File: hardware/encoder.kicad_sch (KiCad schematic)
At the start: 9 parts, among them SW2 PEC12R Encoder

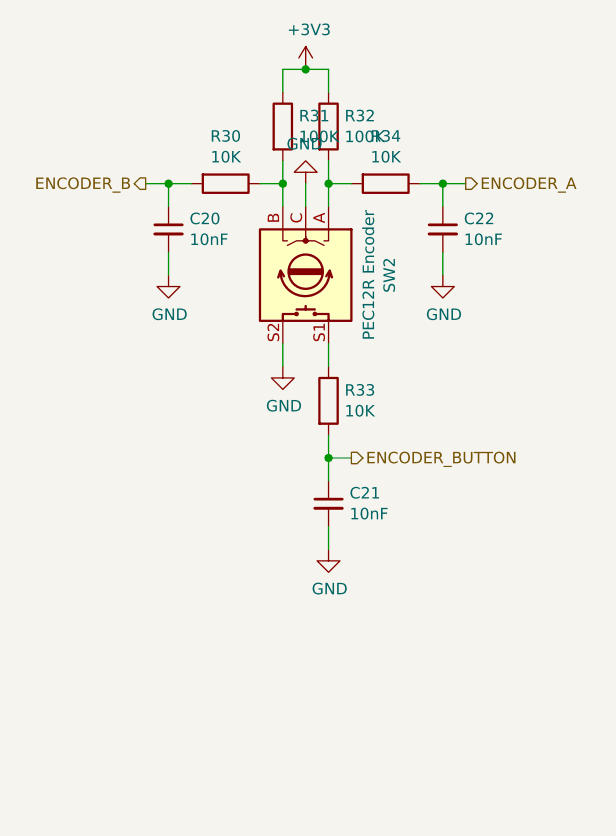
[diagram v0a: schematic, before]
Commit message: Major changes to schematic
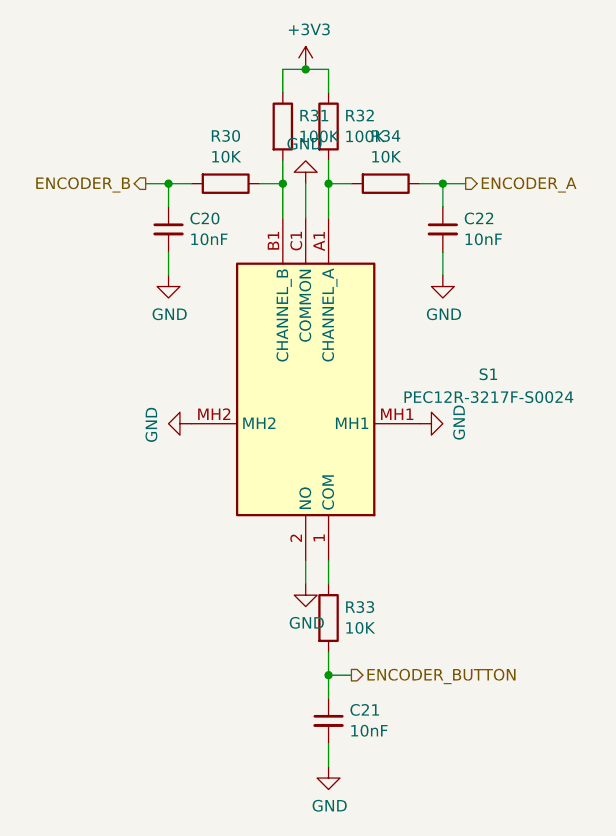
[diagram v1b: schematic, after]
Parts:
- removed SW2: PEC12R Encoder, Custom:Bourns PEC12R Vertical, symbol Device:Rotary_Encoder_Switch
- added S1: PEC12R-3217F-S0024, custom:PEC12R3217FS0024, symbol PEC12R-3217F-S0024:PEC12R-3217F-S0024
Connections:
- net GND: now also S1.2 (NO), S1.C1 (COMMON), S1.MH1, S1.MH2
- net at R32.2, R34.2: now also S1.A1 (CHANNEL_A)
- net at R30.1, R31.2: now also S1.B1 (CHANNEL_B)
- net at R33.1: now also S1.1 (COM)
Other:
- moved on the sheet: C21, R33
